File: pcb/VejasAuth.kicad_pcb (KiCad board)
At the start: 2 copper layers, 18.2 x 45.5 mm, 34 parts, among them J1 USB_A, J3 UP20-C-F-G-FL-P12-TR, SW3 PTS815 SJM 250 SMTR LFS, SW4 PTS815 SJM 250 SMTR LFS, U2 W25Q128JVS, U3 XC6206P332MR-G, U4 RP2350A-QFN60, Y1 ABM8-272-T3

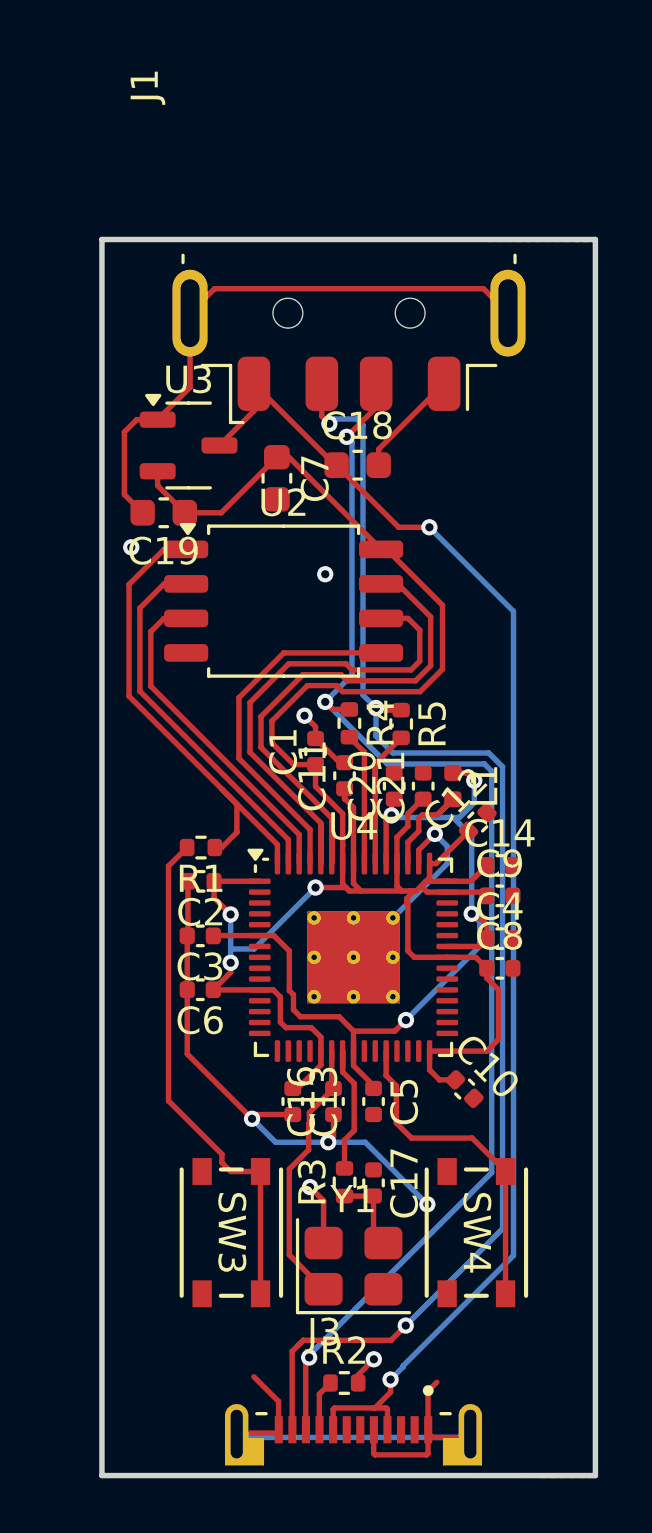
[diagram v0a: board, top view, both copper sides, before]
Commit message: pcb1.1
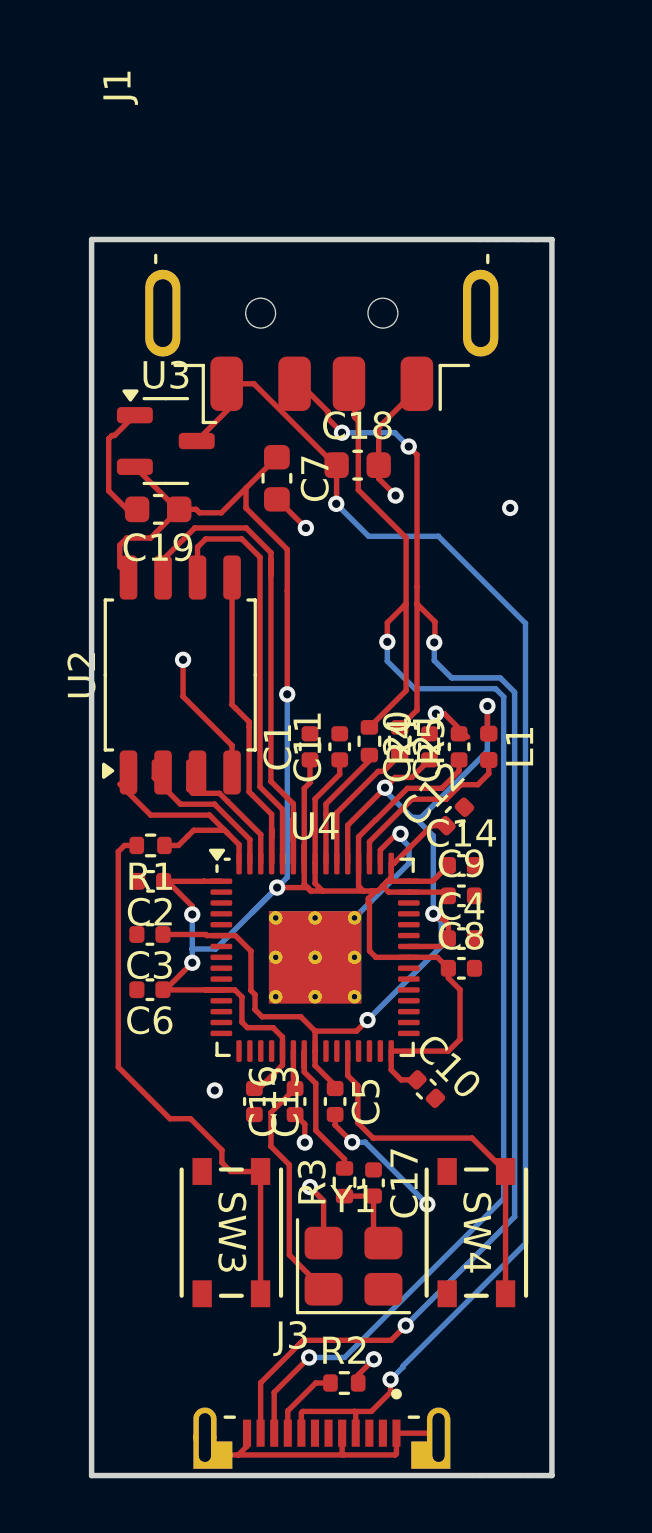
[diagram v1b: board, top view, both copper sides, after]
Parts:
- moved U2 4.68 mm to (158.5, 95.4), turned to 90 degrees
- moved C21 1.96 mm to (168.8, 98.1)
- moved L1 1.96 mm to (169.8, 98.1)
- moved C20 1.94 mm to (167.7, 98.1)
- moved R1 1.86 mm to (157.4, 101.7)
- moved C3 1.85 mm to (157.4, 105.0)
- moved C2 1.85 mm to (157.4, 103.0)
- moved C6 1.85 mm to (157.4, 107.0)
- moved C10 1.41 mm to (167.5, 110.7)
- moved C13 1.41 mm to (161.2, 111.1)
- moved C14 1.41 mm to (168.8, 102.4)
- moved C16 1.41 mm to (162.7, 111.1)
- moved C4 1.41 mm to (168.8, 105.1)
- moved C5 1.41 mm to (164.2, 111.1)
- moved C8 1.41 mm to (168.8, 106.2)
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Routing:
- net GND: track 78.8 -> 46.0 mm, vias 9 -> 12
- net /QSPI_SS: track 18.0 -> 8.58 mm
- net +3V3: track 82.9 -> 90.5 mm, vias 3 -> 4
- net /QSPI_SD1: track 13.7 -> 6.74 mm
- net /QSPI_SD2: track 12.3 -> 5.40 mm
- net +1V1: track 31.7 -> 38.2 mm
- net /D+: track 48.0 -> 52.8 mm, vias 3 -> 2
- net /D-: track 50.6 -> 55.0 mm, vias 3 -> 4
- net /QSPI_SCLK: track 18.3 -> 15.3 mm
- net VBUS: track 50.8 -> 53.5 mm
- net Net-(U4-VREG_LX): track 4.20 -> 6.74 mm
- net Net-(R1-Pad2): track 18.8 -> 20.3 mm
- net /RUN: track 12.1 -> 13.5 mm
- net /QSPI_SD3: track 19.4 -> 20.5 mm
- net Net-(J3-CC1): track 2.01 -> 2.82 mm
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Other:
- board size 18.2 x 45.5 mm -> 16.9 x 45.5 mm
